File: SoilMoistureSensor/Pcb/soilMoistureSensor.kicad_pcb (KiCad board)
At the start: 4 copper layers, 21.3 x 83 mm, 97 parts, among them J1 USB_B_Micro, J2 Conn_01x03, J3 Conn_01x02, J4 Conn_01x03, J5 Conn_01x03, J6 Conn_01x01, J7 Conn_01x01, J8 Conn_01x01, J9 Conn_01x01, U1 W25Q16JVUXIQ, U10 74AUC2G66, U11 TLV9002S, U12 MCP4011-xxxxMS, U2 RP2040, U3 AP63357Q, U4 74AUC2G86, U5 MIC5504-2.5YM5, U6 74AUC2G86, U7 74AUC2G08, U8 OPA2356xxDGK, U9 74AUC2G66, Y1 12Mhz

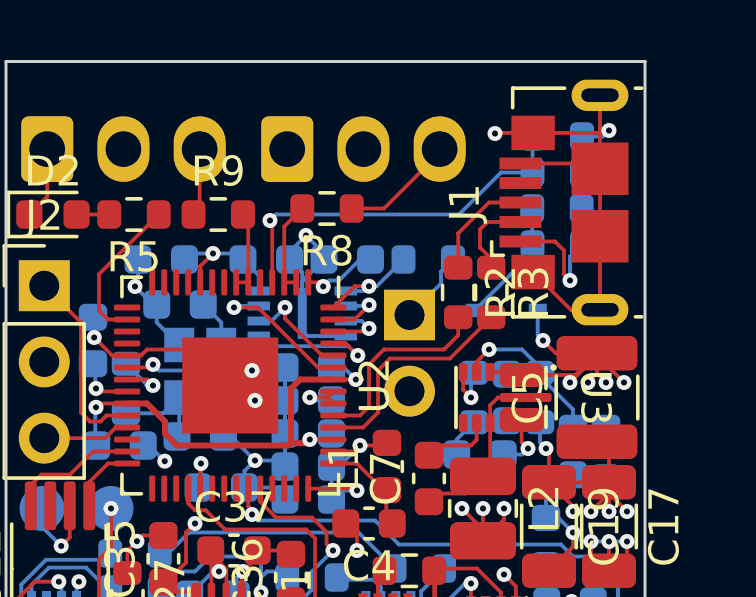
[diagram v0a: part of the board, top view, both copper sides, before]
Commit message: wip
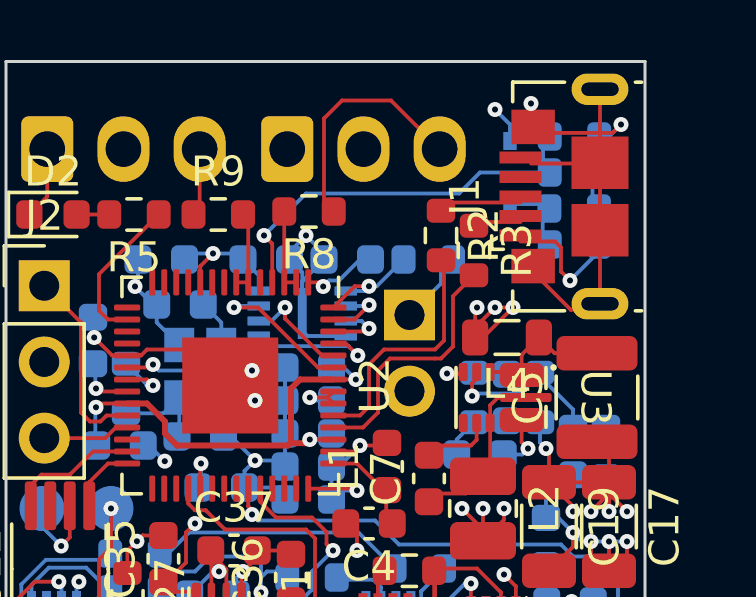
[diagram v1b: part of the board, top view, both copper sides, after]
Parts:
- added L4: 1µ, Inductor_SMD:L_0805_2012Metric, F.Cu at (231.9, 47.6)
- moved D1 4.60 mm to (232.0, 42.1), turned to -90 degrees
- moved R2 1.99 mm to (229.7, 44.2)
- moved R3 1.51 mm to (230.8, 44.7)
- moved R8 0.61 mm to (225.3, 43.4)
- moved R32 0.58 mm to (234.2, 44.5)
- moved R6 0.58 mm to (234.2, 42.1)
- moved R7 0.58 mm to (234.2, 40.9)
- moved R31 0.57 mm to (234.1, 43.3)
- moved J1 0.20 mm to (233.8, 42.9)
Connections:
- C5 pad 2: +24V -> Net-(C5-Pad2)
- U3 pad 1: +24V -> Net-(C5-Pad2)
- U3 pad 2: +24V -> Net-(C5-Pad2)
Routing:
- net +24V: track 11.1 -> 5.83 mm, vias 5 -> 4
- net Net-(C5-Pad2): track 0.00 -> 4.81 mm
- net Net-(J4-Pad3): track 3.82 -> 8.02 mm
- net Net-(R2-Pad2): track 6.69 -> 8.26 mm
- net Net-(D1-Pad2): track 4.20 -> 2.86 mm
- net Net-(J1-Pad2): track 2.88 -> 1.60 mm
- net Net-(R3-Pad2): track 7.60 -> 8.59 mm
- net Net-(J1-Pad3): track 3.65 -> 2.76 mm
- net /UART1: track 3.11 -> 2.26 mm
- net Net-(R6-Pad2): track 12.7 -> 13.3 mm
